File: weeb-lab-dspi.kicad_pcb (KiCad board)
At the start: 2 copper layers, 76.2 x 58.4 mm, 37 parts, among them J1 SPDIF, J2 MONO RCA, J3 AudioJack3_Ground, Q1 BC846, U1 XIAO-RP2350-SMD, U2 MCP130-xxxDxTO, U3 CS8416-xNZ

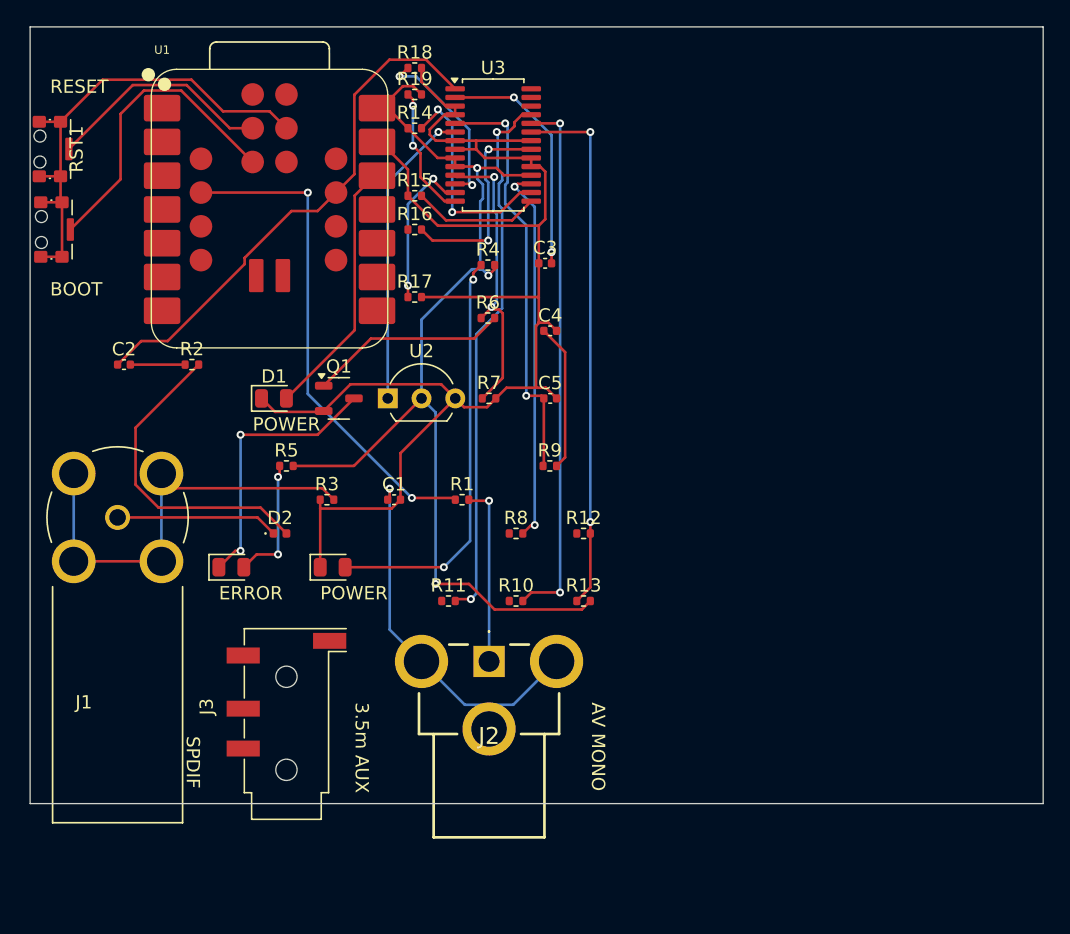
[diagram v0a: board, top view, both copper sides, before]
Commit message: Almost  Complete
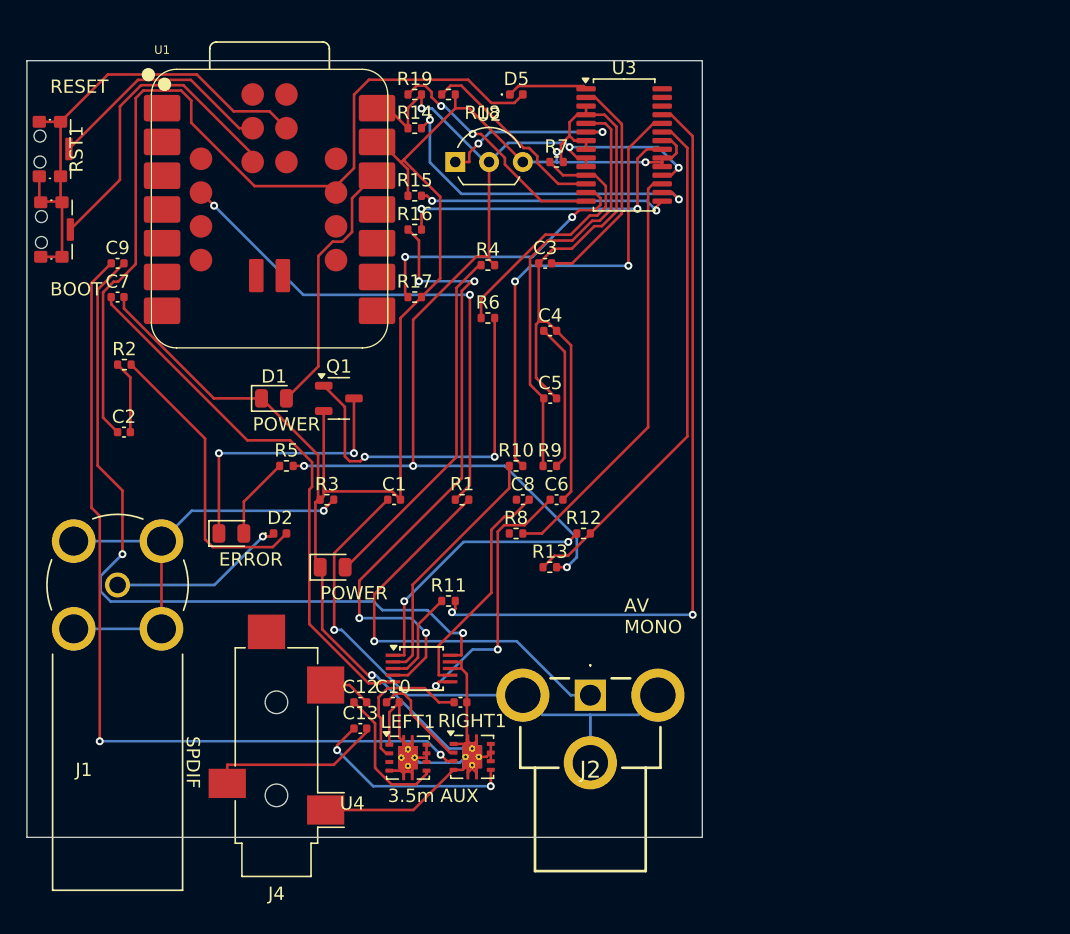
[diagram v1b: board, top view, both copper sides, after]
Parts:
- removed J3: AudioJack3_Ground, Connector_Audio:Jack_3.5mm_KoreanHropartsElec_PJ-320D-4A_Horizontal
- added C10: 0.1uf, Capacitor_SMD:C_0402_1005Metric, F.Cu at (165.5, 99.1)
- added C11: 0.1uf, Capacitor_SMD:C_0402_1005Metric, F.Cu at (170.6, 99.1)
- added C12: 10uf, Capacitor_SMD:C_0402_1005Metric, F.Cu at (163.0, 99.1)
- added C13: 10uf, Capacitor_SMD:C_0402_1005Metric, F.Cu at (163.0, 101.0)
- added C6: 10uf, Capacitor_SMD:C_0402_1005Metric, F.Cu at (177.8, 83.8)
- added C7: 10uf, Capacitor_SMD:C_0402_1005Metric, F.Cu at (144.8, 68.6)
- added C8: 10uf, Capacitor_SMD:C_0402_1005Metric, F.Cu at (175.3, 83.8)
- added C9: 10uf, Capacitor_SMD:C_0402_1005Metric, F.Cu at (144.8, 66.0)
- added D5: BACKFEED_PREVENT, Diode_SMD:D_0402_1005Metric, F.Cu at (174.8, 53.3)
- added J4: AudioJack3_Ground, Connector_Audio:Jack_3.5mm_CUI_SJ-3524-SMT_Horizontal, F.Cu at (156.7, 103.6)
- added LEFT1: TPA6203A1DRB, Package_DFN_QFN:Texas_DRB0008A, F.Cu at (166.6, 103.2)
- added RIGHT1: TPA6203A1DRB, Package_DFN_QFN:Texas_DRB0008A, F.Cu at (171.4, 103.2)
- added U4: CS434x-xZZ, Package_SO:TSSOP-10_3x3mm_P0.5mm, F.Cu at (167.6, 96.5)
- moved R7 18.5 mm to (177.8, 58.4)
- moved U2 18.5 mm to (170.2, 58.4)
- moved R10 10.2 mm to (174.8, 81.3)
- moved U3 9.85 mm to (182.9, 57.1)
- moved J2 8.03 mm to (180.3, 98.5)
- moved R2 5.08 mm to (145.3, 73.7)
- moved C2 5.08 mm to (145.3, 78.7)
- moved J1 5.08 mm to (144.8, 90.2)
- moved R13 3.59 mm to (177.3, 88.9)
- moved R18 3.23 mm to (169.7, 53.3)
- moved D4 2.54 mm to (153.3, 86.4)
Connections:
- C2 pad 1: Net-(U1-GPIO20/D12/TX1) -> Net-(D5-A)
- R10 pad 1: unconnected-(R10-Pad1) -> Net-(U4-~{DEM}/SCLK)
- R11 pad 1: unconnected-(R11-Pad1) -> Net-(U4-LRCK)
- R12 pad 1: unconnected-(R12-Pad1) -> Net-(U4-SDIN)
- R16 pad 1: unconnected-(R16-Pad1) -> Net-(U4-MCLK)
- U1 pad 16: Net-(U1-GPIO20/D12/TX1) -> Net-(D5-A)
- U3 pad 1: Net-(U1-GPIO20/D12/TX1) -> Net-(D5-K)
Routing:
- net GND: track 112.8 -> 222.5 mm, vias 0 -> 3
- net Net-(D5-A): track 0.00 -> 68.1 mm
- net Net-(RIGHT1-IN+): track 0.00 -> 64.1 mm, vias 0 -> 2
- net Net-(U4-AOUTR): track 0.00 -> 58.1 mm, vias 0 -> 2
- net Net-(U4-MCLK): track 0.00 -> 47.8 mm, vias 0 -> 4
- net Net-(U4-VQ): track 0.00 -> 41.0 mm
- net Net-(U1-GPIO20/D12/TX1): track 39.6 -> 0.00 mm
- net Net-(U4-FILT+): track 0.00 -> 20.9 mm, vias 0 -> 2
- net Net-(U4-SDIN): track 0.00 -> 20.0 mm, vias 0 -> 2
- net Net-(U4-~{DEM}/SCLK): track 0.00 -> 18.9 mm
- net Net-(J2-Pad1): track 13.6 -> 31.5 mm
- net Net-(U4-AOUTL): track 0.00 -> 17.2 mm
- net Net-(U3-OLRCK): track 41.0 -> 58.1 mm
- net Net-(RIGHT1-V_{O+}): track 0.00 -> 16.1 mm, vias 0 -> 2
- net Net-(C13-Pad2): track 0.00 -> 13.2 mm
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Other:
- board size 76.2 x 58.4 mm -> 50.8 x 58.4 mm
